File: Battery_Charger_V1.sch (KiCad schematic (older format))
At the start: 98 parts, among them J1 PJ-063AH, J2 Switch, J3 Pad, J4 Pad, J5 Pad, J6 Pad, Q1 IRF4905, Q2 IRF4905, Q3 PSMN4R2_40VSH, Q4 PSMN4R2_40VSH, Q7 2N3904, SW1 (14.4 / 18.0) V Mode Switch, U1 LM7805, U2 LTC3789, U3 MAX713

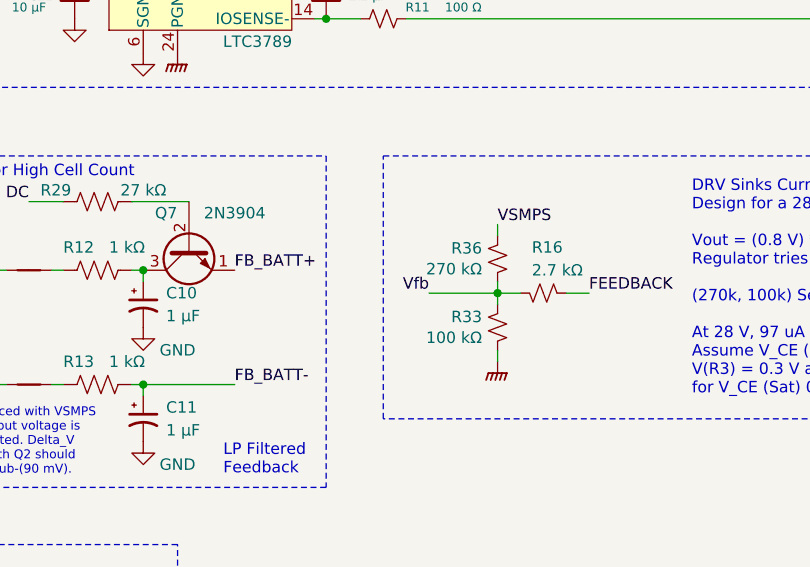
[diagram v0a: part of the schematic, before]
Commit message: Draft PCB(3)
Pre-DRC
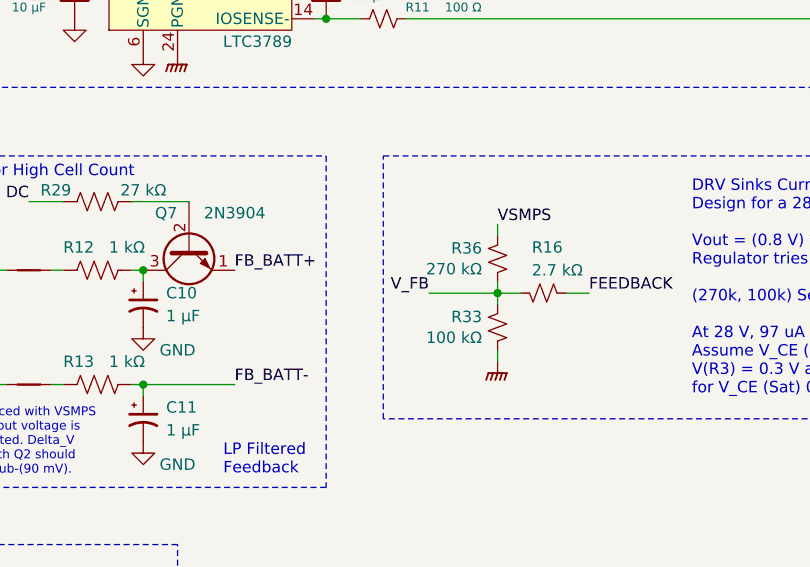
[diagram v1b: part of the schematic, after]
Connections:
- net Vfb is gone; now on net V_FB: R16.2, R33.1, R36.2
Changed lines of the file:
@@
 	7900 4250 7900 4300
 Text Label 7600 4250 2    50   ~ 0
-Vfb
+V_FB
 Text Notes 8750 4700 0    50   ~ 0
 DRV Sinks Current to Increase Voltage\nDesign for a 28 V Max Output\n\nVout = (0.8 V) * (R1 + R2)/(R1)\nRegulator tries to keep Vfb at (0.8 V)\n\n(270k, 100k) Sets a Nominal ~~3 V Target.\n\nAt 28 V, 97 uA across R2.\nAssume V_CE (Sat) 0.5 V,\nV(R3) = 0.3 V at 97 uA --> R3 = 3.1 kOhm\nfor V_CE (Sat) 0.7 V ... R3 = 1.0 kOhm

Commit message: Revised Switch Footprint
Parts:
- Q3, Q4: symbol q_dual_nmos_psmn4r2_40vsh:Q_DUAL_NMOS_PSMN4R2_40VSH -> Battery_Charger_V1-rescue:Q_DUAL_NMOS_PSMN4R2_40VSH-q_dual_nmos_psmn4r2_40vsh
- SW1: footprint Button_Switch_THT:SW_E-Switch_EG1271_DPDT -> CK_Switches:DPDT
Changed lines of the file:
@@
 F 0 "SW1" H 5950 6300 50  0000 C CNN
 F 1 "(14.4 / 18.0) V Mode Switch" H 6000 5450 50  0000 C CNN
-F 2 "Button_Switch_THT:SW_E-Switch_EG1271_DPDT" H 5950 6100 50  0001 C CNN
+F 2 "CK_Switches:DPDT" H 5950 6100 50  0001 C CNN
 F 3 "~" H 5950 6100 50  0001 C CNN
 	1    5950 5900
@@
 	8300 2400 8250 2400
 $Comp
-L q_dual_nmos_psmn4r2_40vsh:Q_DUAL_NMOS_PSMN4R2_40VSH Q3
+L Battery_Charger_V1-rescue:Q_DUAL_NMOS_PSMN4R2_40VSH-q_dual_nmos_psmn4r2_40vsh Q3
 U 1 1 6375112D
 P 8075 1450
@@
 $EndComp
 $Comp
-L q_dual_nmos_psmn4r2_40vsh:Q_DUAL_NMOS_PSMN4R2_40VSH Q3
+L Battery_Charger_V1-rescue:Q_DUAL_NMOS_PSMN4R2_40VSH-q_dual_nmos_psmn4r2_40vsh Q3
 U 2 1 6375262B
 P 8075 1850
@@
 	8100 1650 8175 1650
 $Comp
-L q_dual_nmos_psmn4r2_40vsh:Q_DUAL_NMOS_PSMN4R2_40VSH Q4
+L Battery_Charger_V1-rescue:Q_DUAL_NMOS_PSMN4R2_40VSH-q_dual_nmos_psmn4r2_40vsh Q4
 U 1 1 63775358
 P 9250 1450
@@
 $EndComp
 $Comp
-L q_dual_nmos_psmn4r2_40vsh:Q_DUAL_NMOS_PSMN4R2_40VSH Q4
+L Battery_Charger_V1-rescue:Q_DUAL_NMOS_PSMN4R2_40VSH-q_dual_nmos_psmn4r2_40vsh Q4
 U 2 1 63775F64
 P 9250 1850
